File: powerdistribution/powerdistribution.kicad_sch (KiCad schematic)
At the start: 110 parts, among them IC1 STEF01FTR, IC2 STEF01FTR, IC3 STEF01FTR, J1 282837-2, J2 282837-2, J3 M20-6102045, J4 Screw_Terminal_01x02, J5 Screw_Terminal_01x02, Q1 IRLML0030, Q2 IRLML0030, Q3 IRLML0030, Q4 SI4925DDY-T1-GE3, Q5 IRLML0030, SW1 RA1H1C112R, SW2 RA1H1C112R, U1 BQ7790512PW, U2 AP64501QSP-13, U3 AP64501QSP-13, U4 AP64501QSP-13

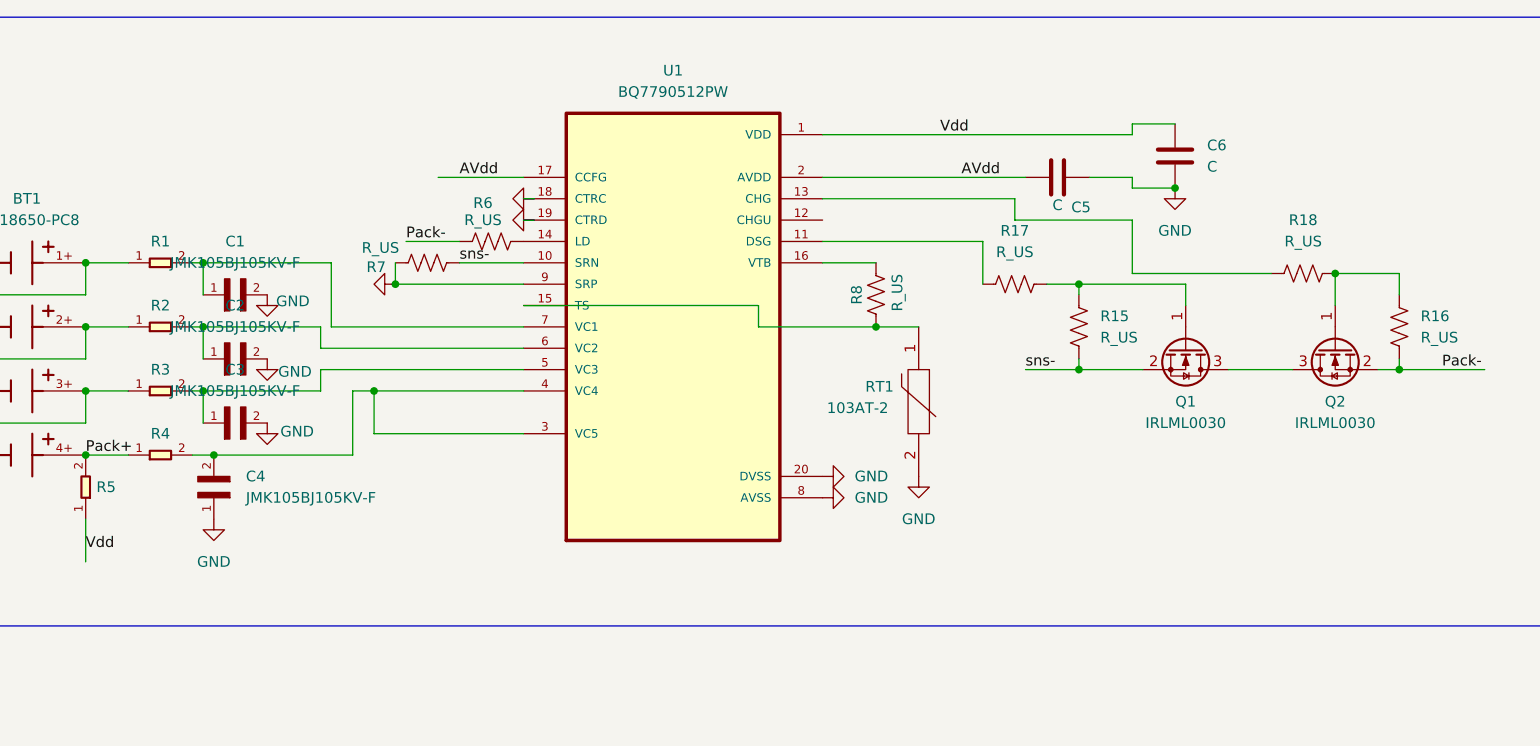
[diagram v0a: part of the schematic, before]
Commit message: add models
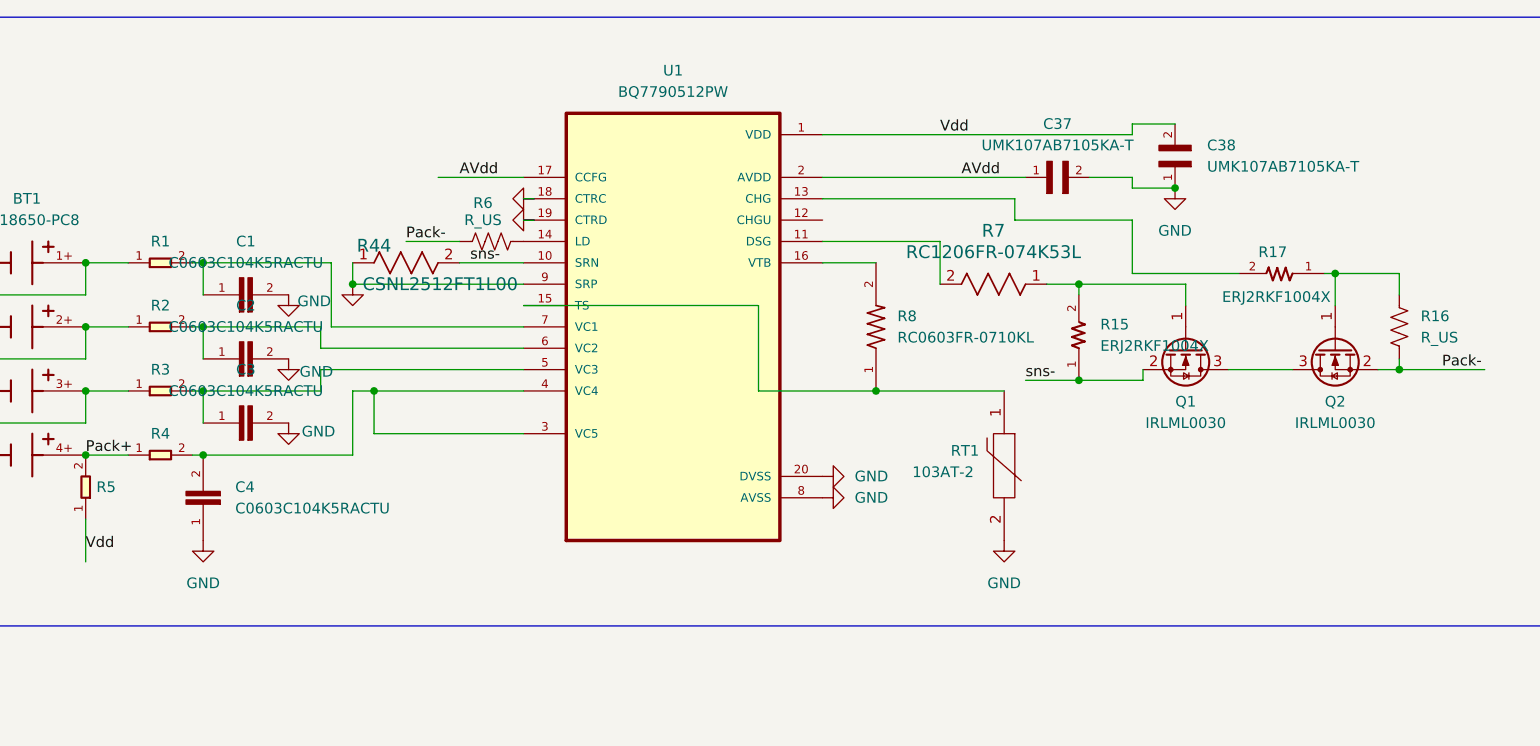
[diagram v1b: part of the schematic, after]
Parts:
- removed C1, C2, C3, C4: JMK105BJ105KV-F, HPRfootprints:CAPC1005X55N, symbol HPRsymbols:JMK105BJ105KV-F
- removed C5, C6: C, symbol Device:C
- removed R15, R17, R18, R7, R8: R_US, symbol Device:R_US
- added C1, C2, C3, C4: C0603C104K5RACTU, C0603C104K5RACTU:CAPC1608X90, symbol HPRsymbols:C0603C104K5RACTU
- added C37, C38: UMK107AB7105KA-T, UMK107AB7105KA-T:CAPC1608X95N, symbol HPRsymbols:UMK107AB7105KA-T
- added R15, R17: ERJ2RKF1004X, ERJ2RKF1004X:RES_ERJ2RKF1004X, symbol HPRsymbols:ERJ2RKF1004X
- added R44: CSNL2512FT1L00, STA_CSNL25121_STP, symbol HPRsymbols:CSNL2512FT1L00
- added R7: RC1206FR-074K53L, RC1206N_YAG, symbol HPRsymbols:RC1206FR-074K53L
- added R8: RC0603FR-0710KL, RC0603FR-0710KL:RESC1607X60N, symbol HPRsymbols:RC0603FR-0710KL
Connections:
- net AVdd: now also C37.1
- net GND: now also C1.2, C2.2, C3.2, C37.2, C38.1, C4.1, R44.1
- net Vdd: now also C38.2
- net sns-: now also R15.1, R44.2
- net at R4.2, U1.3 (VC5), U1.4 (VC4): now also C4.2
- net at Q2.1 (G), R16.1: now also R17.1
- net at RT1.1, U1.15 (TS): now also R8.1
- net at U1.16 (VTB): now also R8.2
- net at U1.13 (CHG): now also R17.2
- net at U1.11 (DSG): now also R7.2
- net at R3.2, U1.5 (VC3): now also C3.1
- net at R2.2, U1.6 (VC2): now also C2.1
- net at R1.2, U1.7 (VC1): now also C1.1
- net at Q1.1 (G): now also R15.2, R7.1
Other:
- moved on the sheet: RT1
